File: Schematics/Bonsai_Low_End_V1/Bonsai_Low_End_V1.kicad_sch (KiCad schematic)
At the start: 24 parts, among them J1 Bat_Connector, Q1 PMOS, U1 MOUDLE-SEEEDUINO-XIAO-ESP32C3, U2 MAX30101EFD, U3 1.8V, U5 DRV2605LDGS

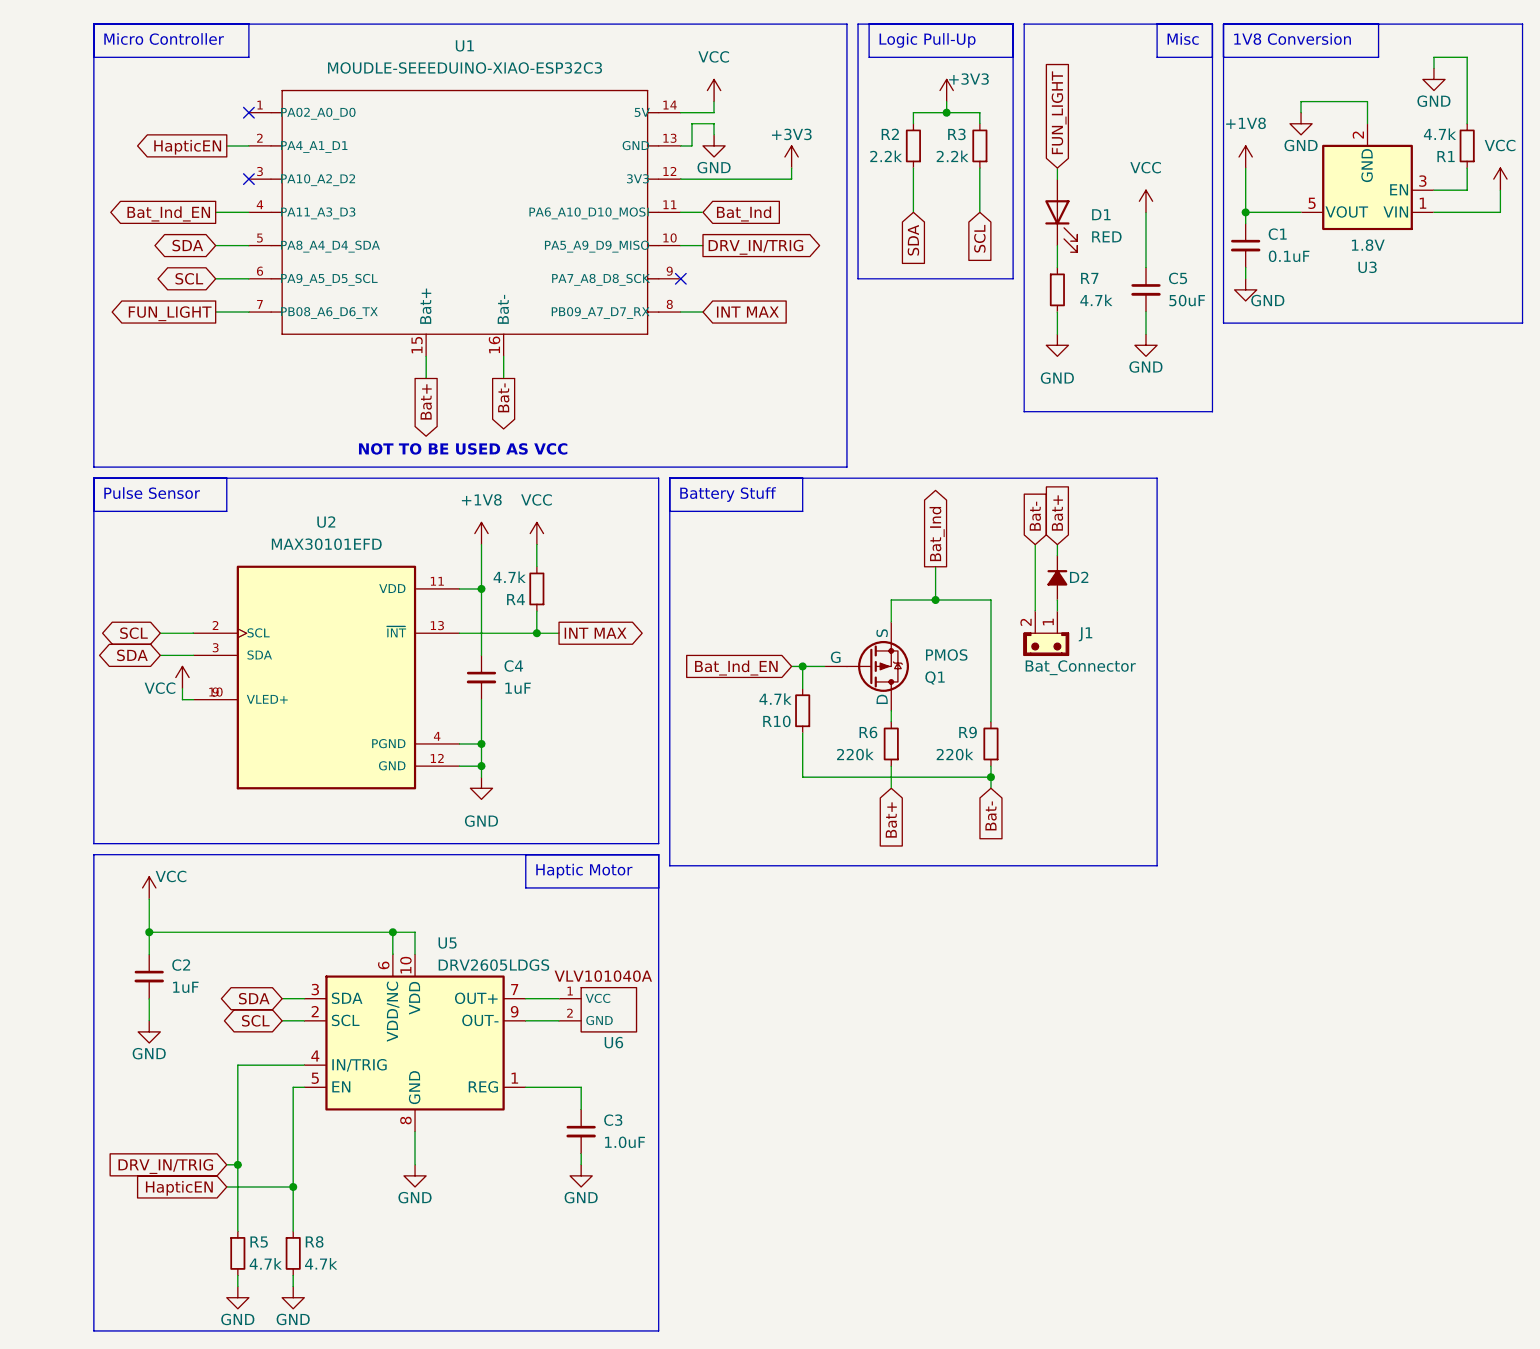
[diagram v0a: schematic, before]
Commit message: prior symbol change
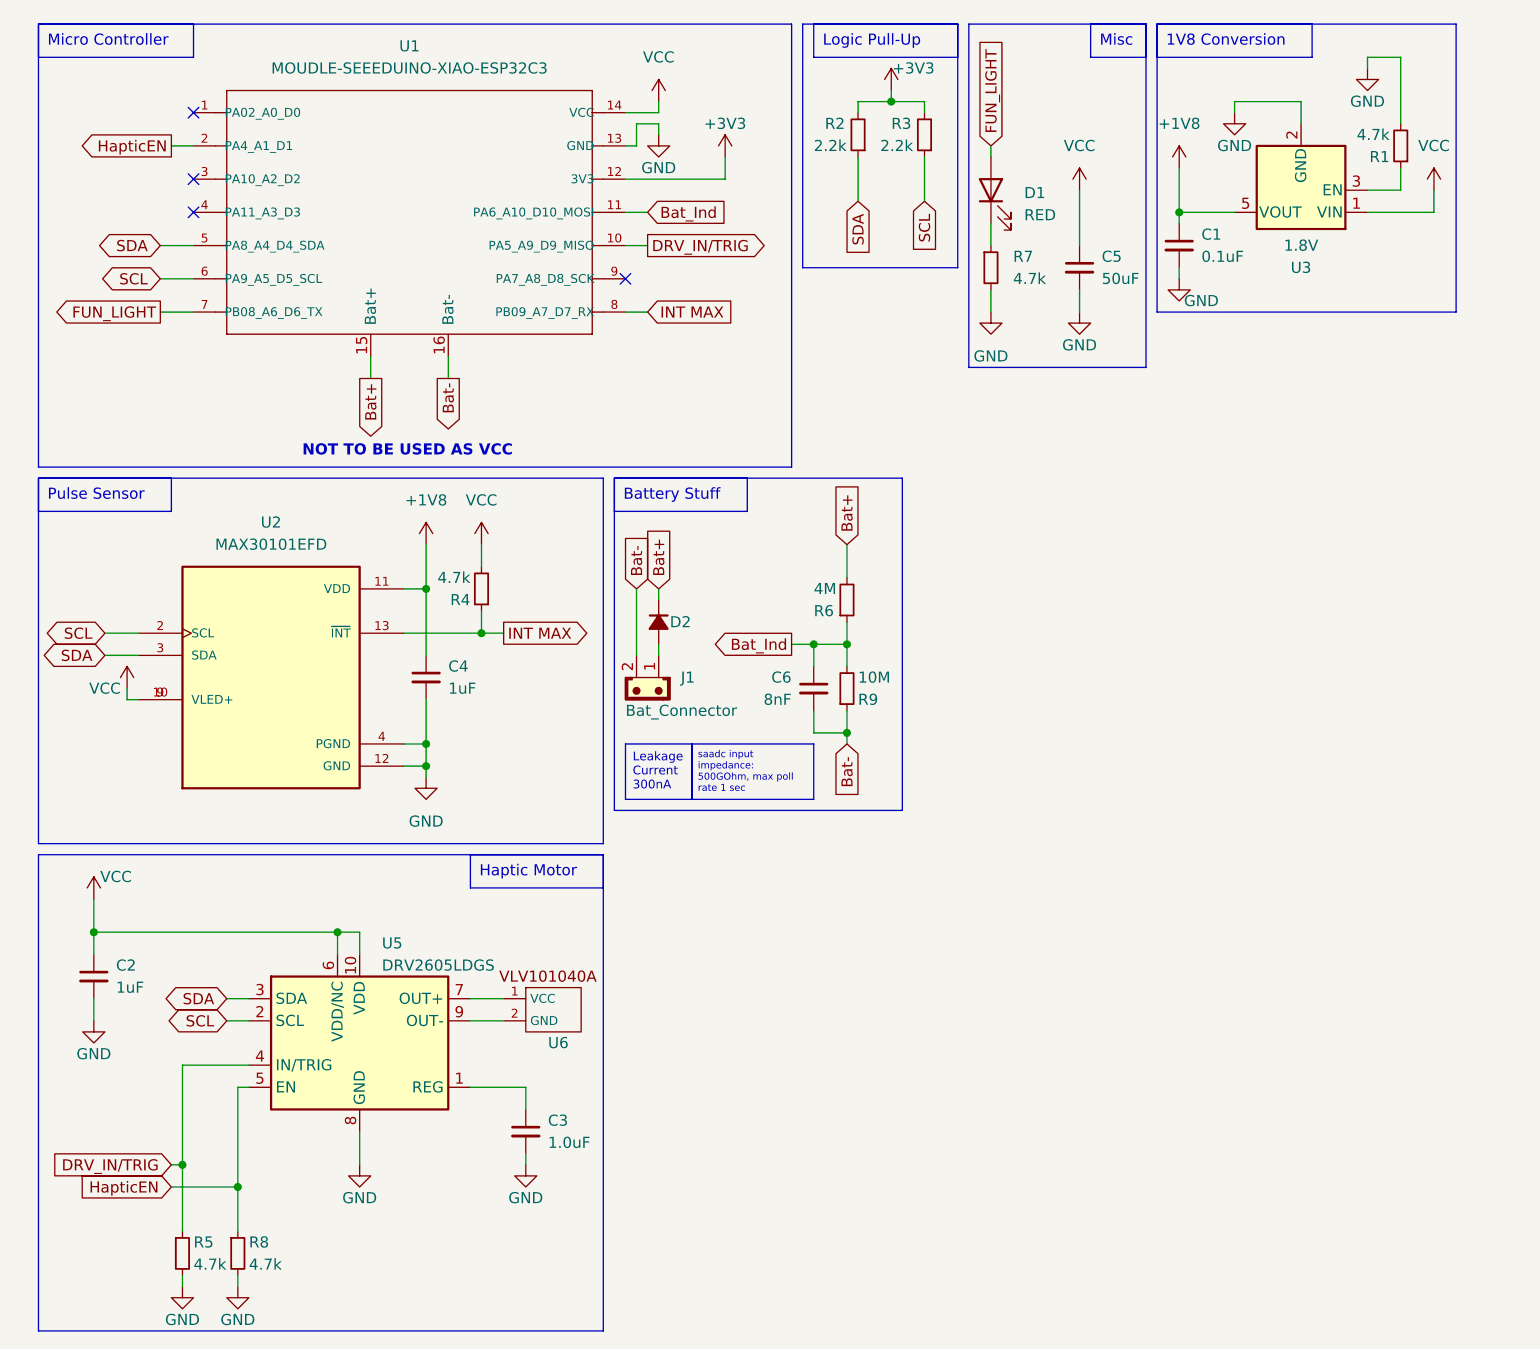
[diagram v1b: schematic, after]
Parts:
- removed Q1: PMOS, symbol Simulation_SPICE:PMOS
- removed R10: 4.7k, Resistor_SMD:R_0603_1608Metric_Pad0.98x0.95mm_HandSolder, symbol Device:R_Small
- added C6: 8nF, Capacitor_SMD:C_0805_2012Metric_Pad1.18x1.45mm_HandSolder, symbol Device:C_Small
- R6: value 220k -> 4M
- R9: value 220k -> 10M
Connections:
- net Bat+: now also R6.2; no longer R6.1
- net Bat-: now also C6.2
- net Bat_Ind: now also R6.1, C6.1
- net Bat_Ind_EN: no longer names the net of U1.4 (PA11_A3_D3)
- no-connect marks 3 -> 4
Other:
- moved on the sheet: C1, C2, C3, C4, C5, D1, D2, J1, R1, R2, R3, R4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
